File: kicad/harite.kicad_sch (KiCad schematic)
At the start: 10 parts, among them J1 503480-0500, J2 5034801000, J3 5034801000, U3 Raspberry_Pi_Pico

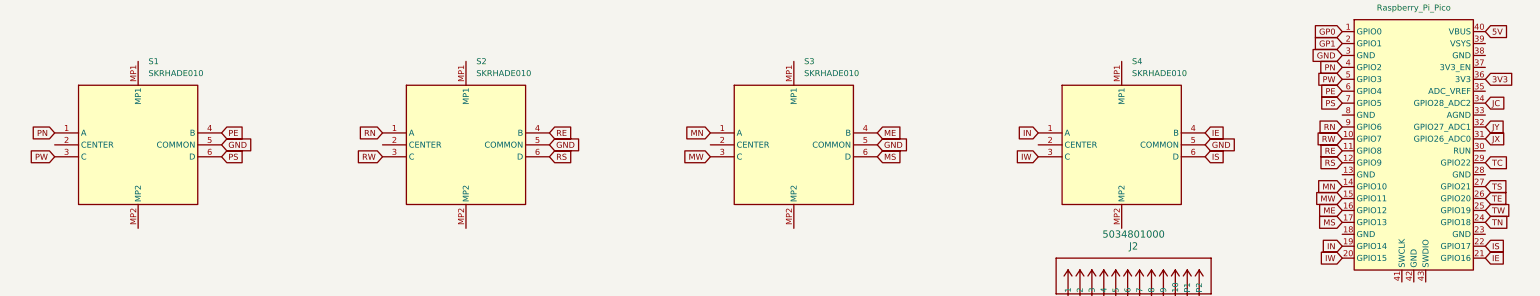
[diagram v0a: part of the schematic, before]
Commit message: update
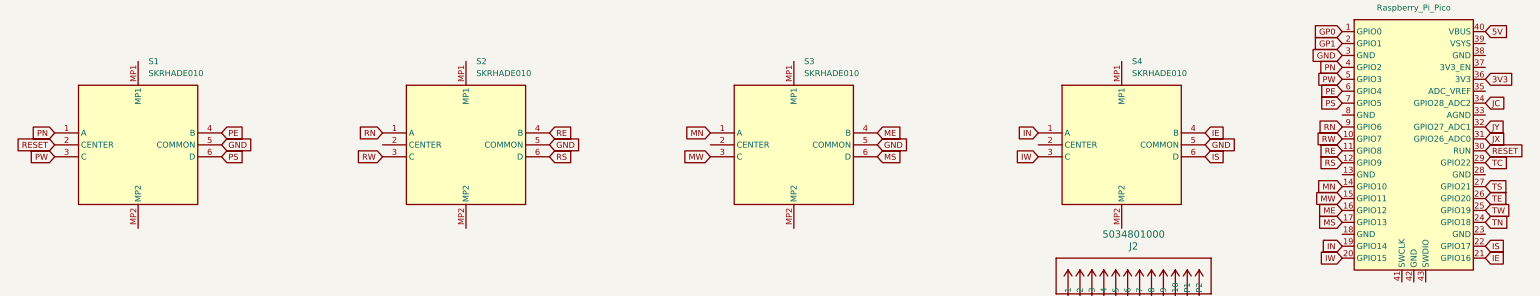
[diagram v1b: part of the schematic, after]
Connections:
- net RESET: now reaches S1.2 (CENTER)
- net RESET: now also U3.30 (RUN)
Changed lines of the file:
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@@
+		)
+	)
+	(global_label "RESET"
+		(shape input)
+		(at 332.74 59.69 0)
+		(fields_autoplaced yes)
+		(effects
+			(font
+				(size 1.27 1.27)
+			)
+			(justify left)
+		)
+		(property "Intersheetrefs" "${INTERSHEET_REFS}"
+			(at 341.4703 59.69 0)
+			(effects
+				(font
+					(size 1.27 1.27)
+				)
+				(justify left)
+				(hide yes)
+			)
 		)
 	)
@@
 			(effects
 				(font
+					(size 1.27 1.27)
+				)
+				(justify right)
+				(hide yes)
+			)
+		)
+	)
+	(global_label "RESET"
+		(shape input)
+		(at 27.94 58.42 180)
+		(fields_autoplaced yes)
+		(effects
+			(font
+				(size 1.27 1.27)
+			)
+			(justify right)
+		)
+		(property "Intersheetrefs" "${INTERSHEET_REFS}"
+			(at 19.2097 58.42 0)
+			(effects
+				(font
